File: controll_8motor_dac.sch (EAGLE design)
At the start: 61 parts

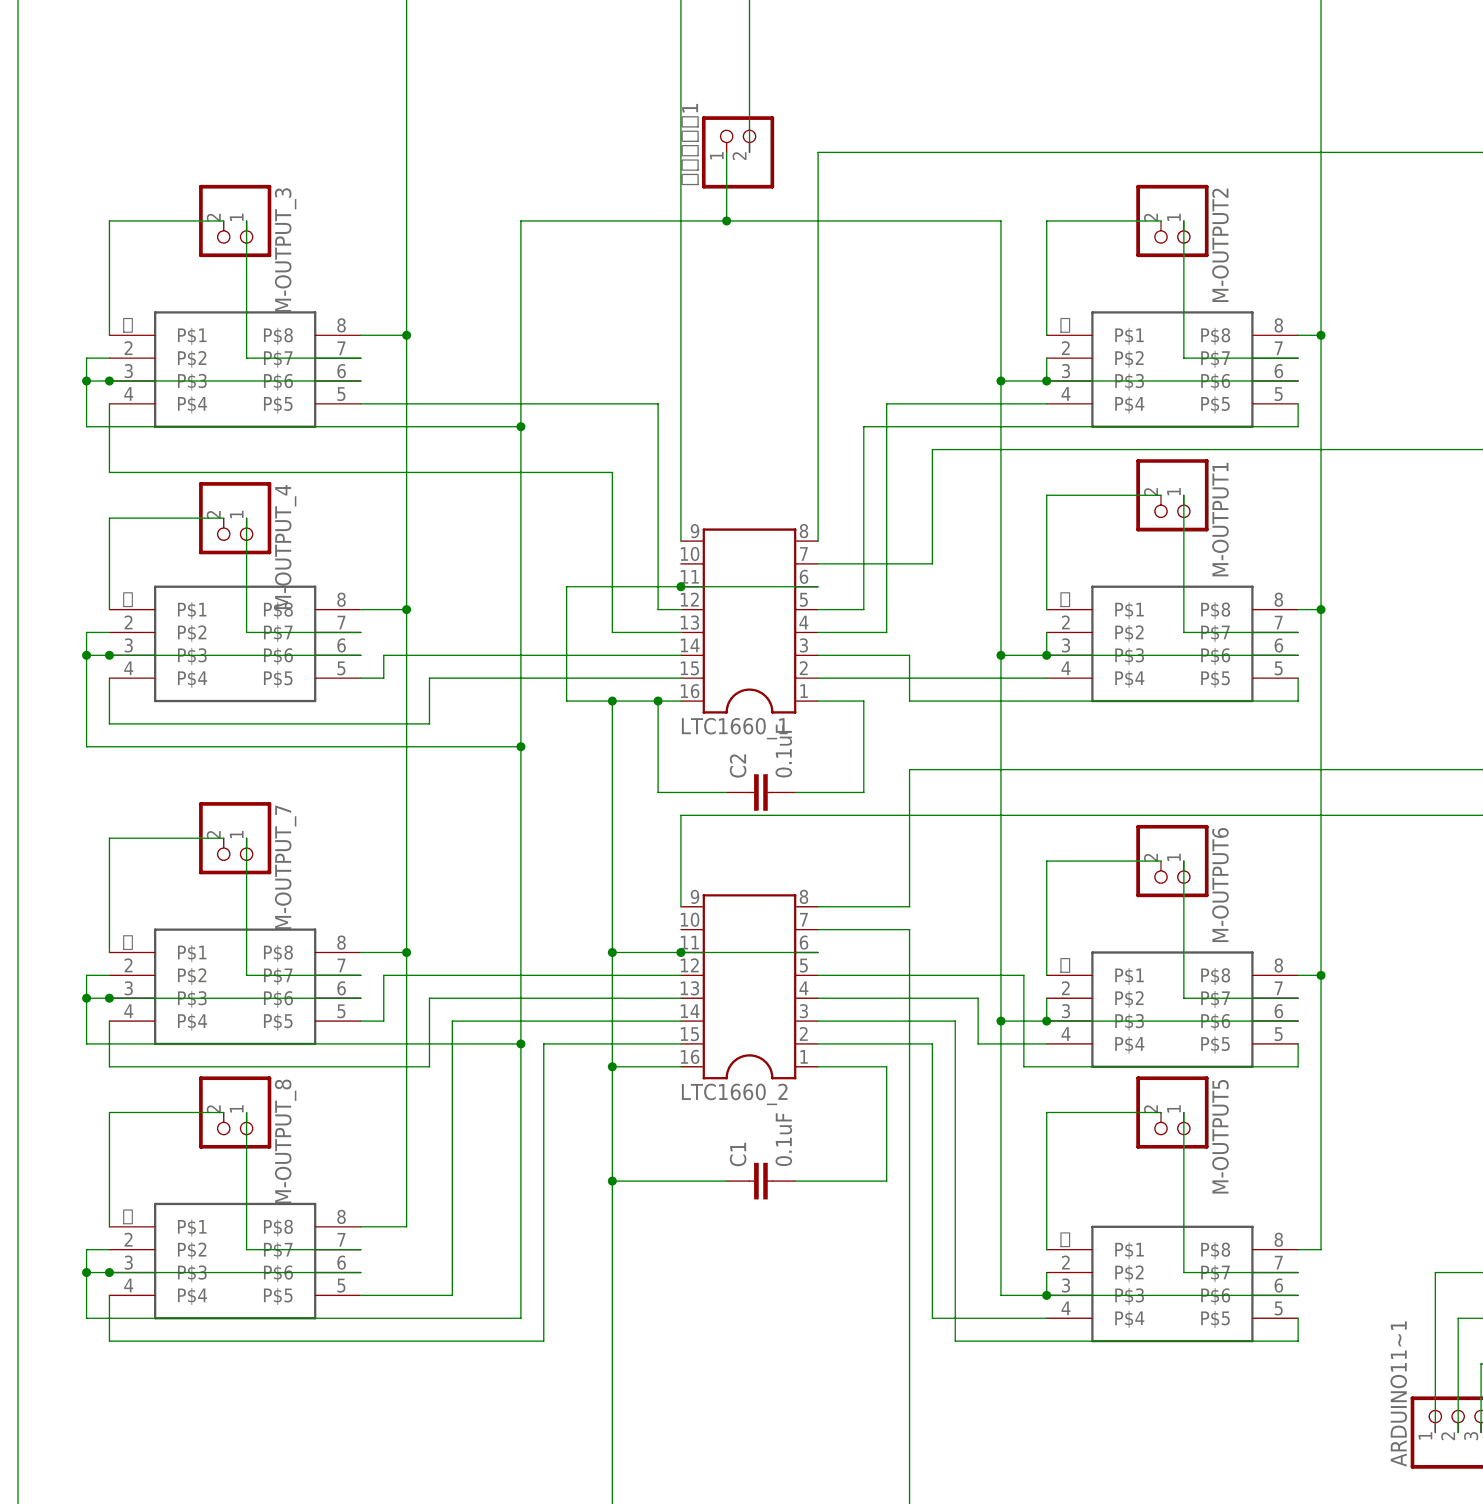
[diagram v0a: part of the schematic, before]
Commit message: 配線してみた,icパーツ使ってみた
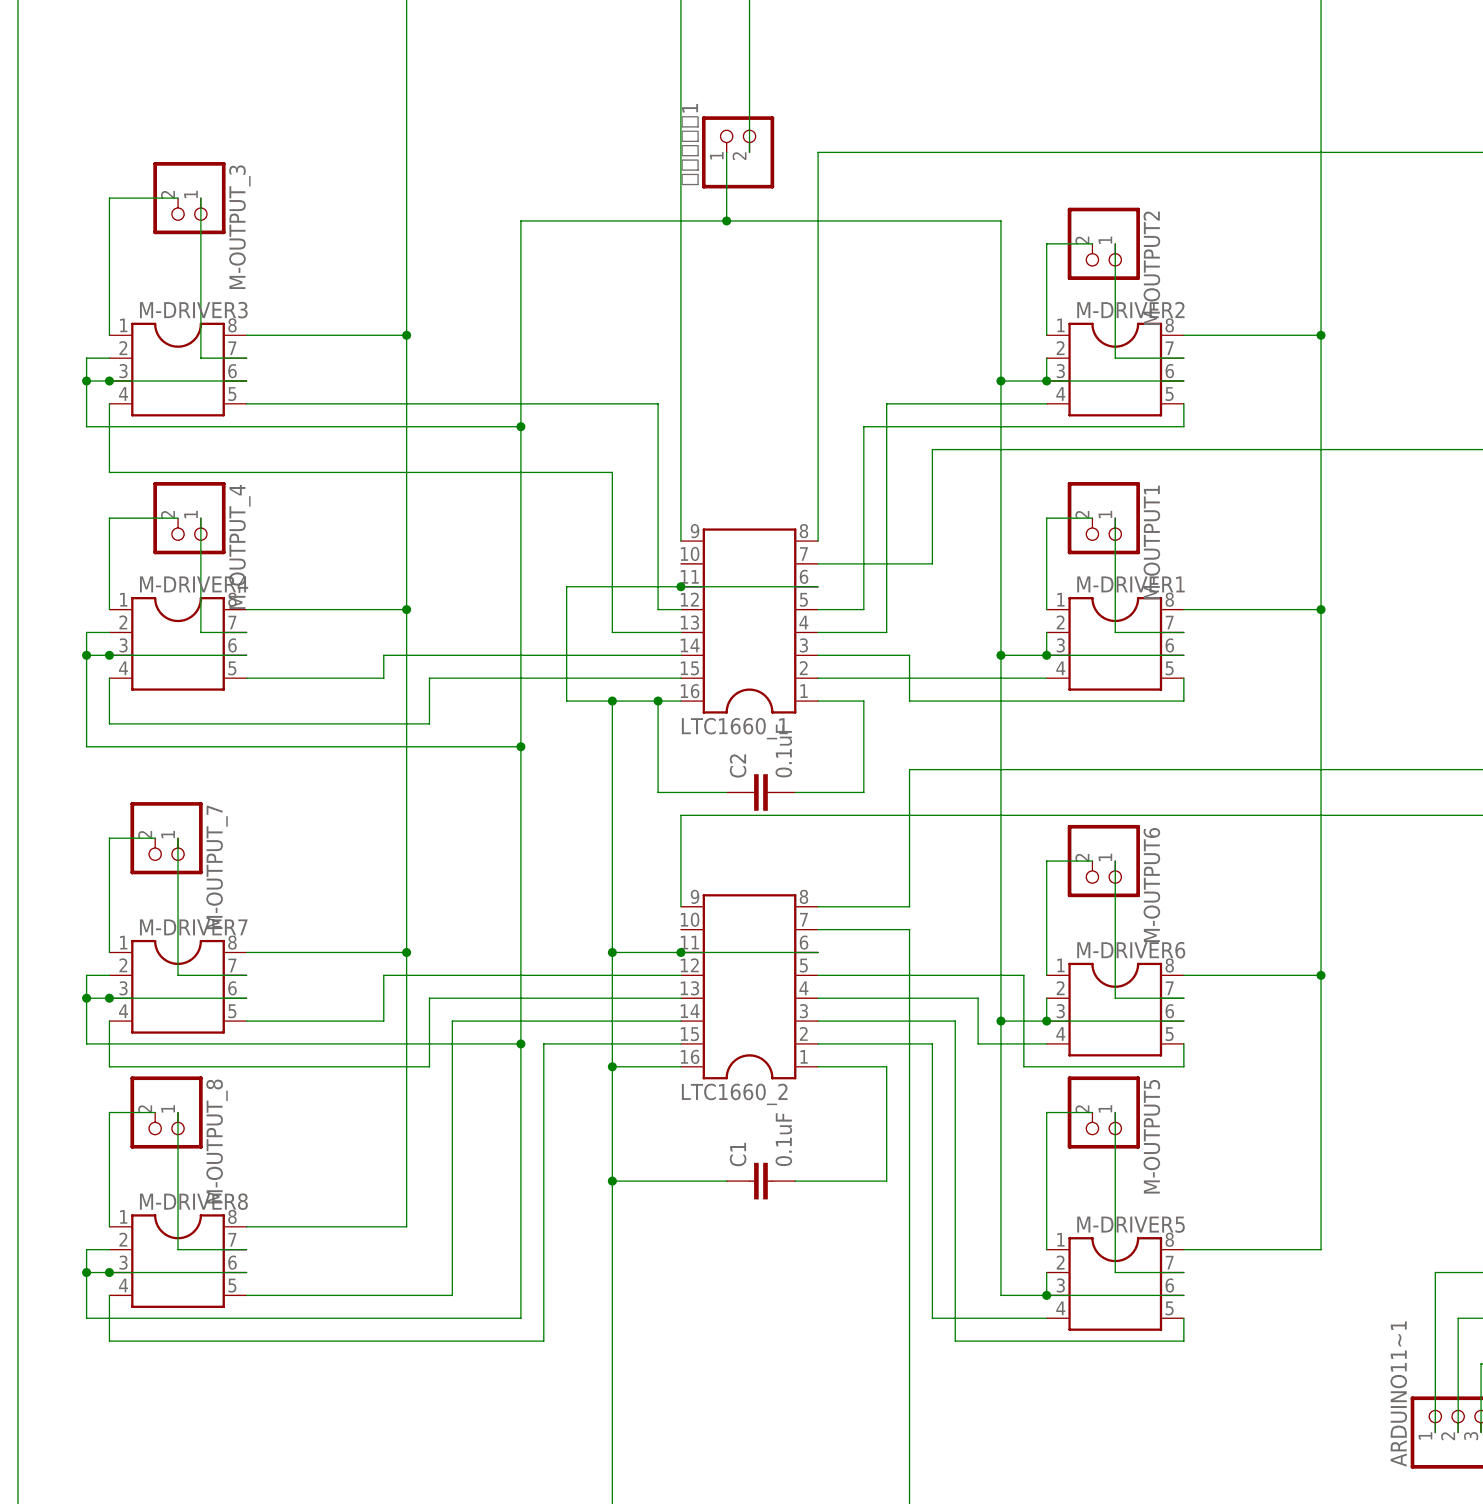
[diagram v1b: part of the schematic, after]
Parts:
- M-DRIVER1, M-DRIVER2, M-DRIVER3, M-DRIVER4, M-DRIVER5, M-DRIVER6, M-DRIVER7, M-DRIVER8: value SOP8-DIP-CONVERTER -> (none); device SOP8-DIP-Converter:SOP8-DIP-CONVERTER -> ic-package:DIL8S
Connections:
- net N$1: now also M-DRIVER3.5; no longer M-DRIVER3.P$5
- net N$10: now also M-DRIVER2.4; no longer M-DRIVER2.P$4
- net N$11: now also M-DRIVER1.5; no longer M-DRIVER1.P$5
- net N$12: now also M-DRIVER1.4; no longer M-DRIVER1.P$4
- net N$13: now also M-DRIVER5.1; no longer M-DRIVER5.P$1
- net N$14: now also M-DRIVER6.4; no longer M-DRIVER6.P$4
- net N$15: now also M-DRIVER5.5; no longer M-DRIVER5.P$5
- net N$16: now also M-DRIVER5.4; no longer M-DRIVER5.P$4
- net N$17: now also M-DRIVER3.7; no longer M-DRIVER3.P$7
- net N$18: now also M-DRIVER4.7; no longer M-DRIVER4.P$7
- net N$19: now also M-DRIVER4.1; no longer M-DRIVER4.P$1
- net N$2: now also M-DRIVER3.1; no longer M-DRIVER3.P$1
- net N$20: now also M-DRIVER7.7; no longer M-DRIVER7.P$7
- net N$21: now also M-DRIVER7.1; no longer M-DRIVER7.P$1
- net N$22: now also M-DRIVER8.7; no longer M-DRIVER8.P$7
- net N$23: now also M-DRIVER8.1; no longer M-DRIVER8.P$1
- net N$24: now also M-DRIVER1.7; no longer M-DRIVER1.P$7
- net N$26: now also M-DRIVER4.5; no longer M-DRIVER4.P$5
- net N$27: now also M-DRIVER2.7; no longer M-DRIVER2.P$7
- net N$28: now also M-DRIVER2.1; no longer M-DRIVER2.P$1
- net N$29: now also M-DRIVER6.5; no longer M-DRIVER6.P$5
- net N$3: now also M-DRIVER3.4; no longer M-DRIVER3.P$4
- net N$30: now also M-DRIVER5.7; no longer M-DRIVER5.P$7
- net N$31: now also M-DRIVER6.1; no longer M-DRIVER6.P$1
- net N$32: now also M-DRIVER6.7; no longer M-DRIVER6.P$7
- net N$33: now also M-DRIVER1.2, M-DRIVER1.3, M-DRIVER1.6, M-DRIVER2.2, M-DRIVER2.3, M-DRIVER2.6, M-DRIVER3.2, M-DRIVER3.3, M-DRIVER3.6, M-DRIVER4.2, M-DRIVER4.3, M-DRIVER4.6, M-DRIVER5.2, M-DRIVER5.3, M-DRIVER5.6, M-DRIVER6.2, M-DRIVER6.3, M-DRIVER6.6, M-DRIVER7.2, M-DRIVER7.3, M-DRIVER7.6, M-DRIVER8.2, M-DRIVER8.3, M-DRIVER8.6; no longer M-DRIVER1.P$2, M-DRIVER1.P$3, M-DRIVER1.P$6, M-DRIVER2.P$2, M-DRIVER2.P$3, M-DRIVER2.P$6, M-DRIVER3.P$2, M-DRIVER3.P$3, M-DRIVER3.P$6, M-DRIVER4.P$2, M-DRIVER4.P$3, M-DRIVER4.P$6, M-DRIVER5.P$2, M-DRIVER5.P$3, M-DRIVER5.P$6, M-DRIVER6.P$2, M-DRIVER6.P$3, M-DRIVER6.P$6, M-DRIVER7.P$2, M-DRIVER7.P$3, M-DRIVER7.P$6, M-DRIVER8.P$2, M-DRIVER8.P$3, M-DRIVER8.P$6
- net N$4: now also M-DRIVER4.4; no longer M-DRIVER4.P$4
- net N$40: now also M-DRIVER1.1; no longer M-DRIVER1.P$1
- net N$5: now also M-DRIVER7.5; no longer M-DRIVER7.P$5
- net N$6: now also M-DRIVER7.4; no longer M-DRIVER7.P$4
- net N$7: now also M-DRIVER8.5; no longer M-DRIVER8.P$5
- net N$8: now also M-DRIVER8.4; no longer M-DRIVER8.P$4
- net N$9: now also M-DRIVER2.5; no longer M-DRIVER2.P$5
- net P-DIORD1: now also M-DRIVER1.8, M-DRIVER2.8, M-DRIVER3.8, M-DRIVER4.8, M-DRIVER5.8, M-DRIVER6.8, M-DRIVER7.8, M-DRIVER8.8; no longer M-DRIVER1.P$8, M-DRIVER2.P$8, M-DRIVER3.P$8, M-DRIVER4.P$8, M-DRIVER5.P$8, M-DRIVER6.P$8, M-DRIVER7.P$8, M-DRIVER8.P$8
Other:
- moved on the sheet: M-OUTPUT1, M-OUTPUT2, M-OUTPUT5, M-OUTPUT6, M-OUTPUT_3, M-OUTPUT_4, M-OUTPUT_7, M-OUTPUT_8
